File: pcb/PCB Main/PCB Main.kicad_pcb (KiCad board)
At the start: 4 copper layers, 64.1 x 56.5 mm, 82 parts, among them CN1 Conn_01x07, CN2 Conn_01x02, CN3 Conn_01x02, CN4 Conn_01x04, CN5 Conn_01x04, CN6 Conn_01x03, CN7 Conn_01x03, CN8 Conn_01x03, CN9 Conn_01x02, J1 Conn_01x03, Q1 AO3401A, SW1 SW_Reset, U1 STM32WB55RGVx, U2 AEM10941, U3 INA3221, U4 MB85RS256B, X1 32MHz, X2 32.768kHz

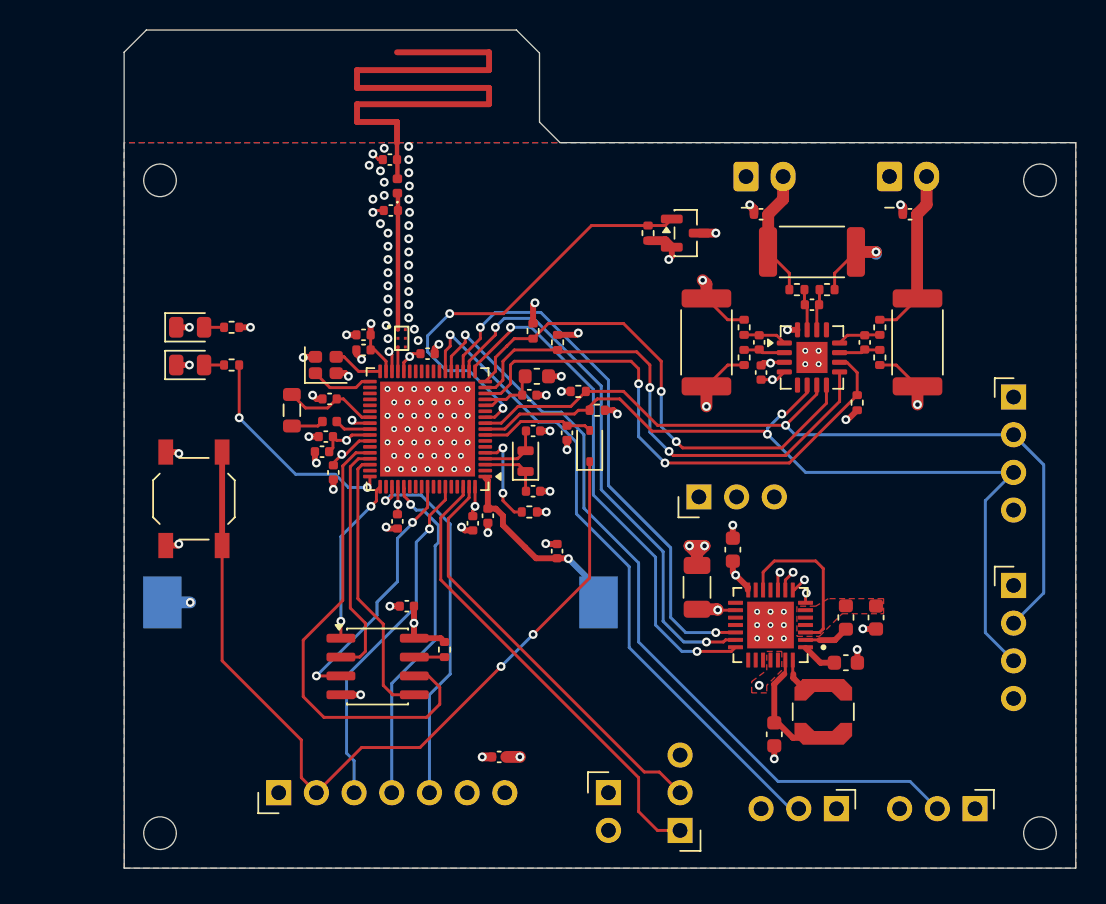
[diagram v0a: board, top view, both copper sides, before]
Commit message: islas cristales
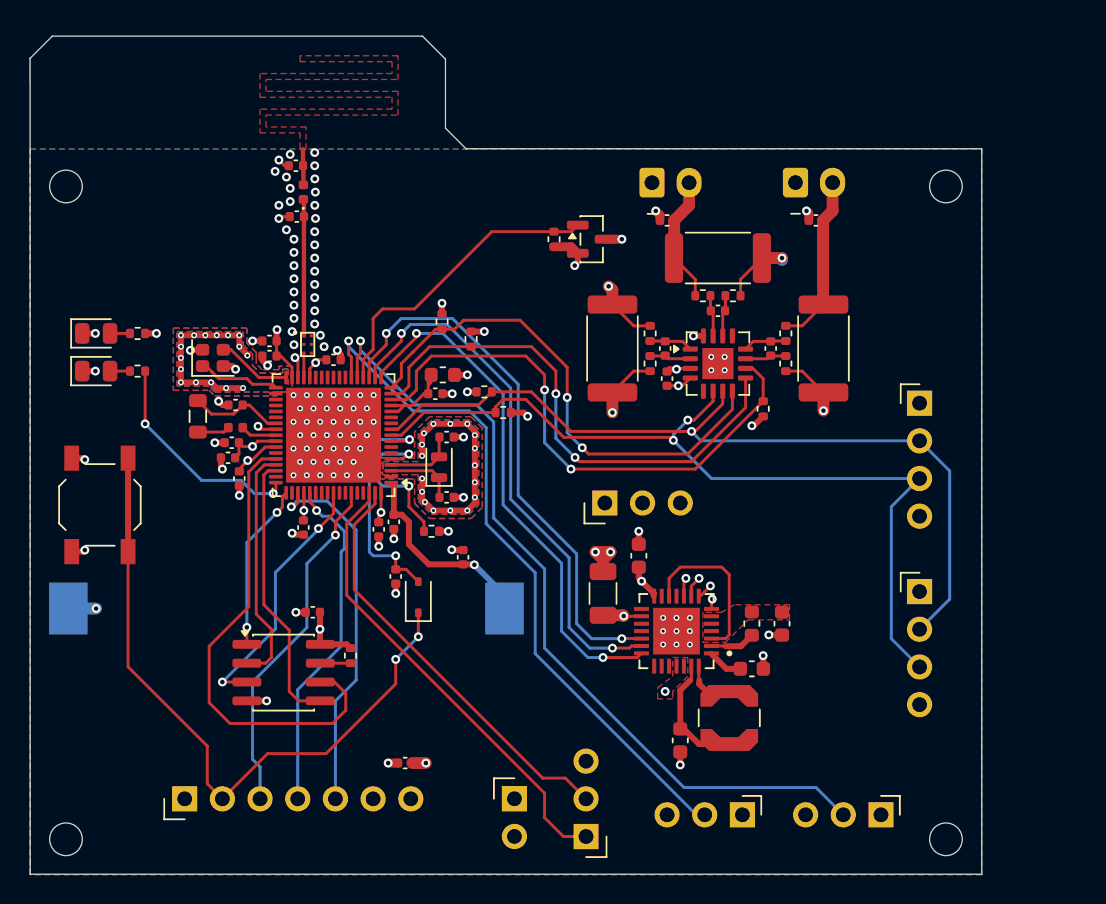
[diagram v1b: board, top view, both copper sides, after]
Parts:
- moved D1 15.4 mm to (41.0, 52.2)
- moved C23 15.1 mm to (39.5, 50.8)
- moved X1 7.62 mm to (27.2, 36.1)
- moved R13 6.72 mm to (41.9, 47.8)
- moved C18 6.35 mm to (33.3, 47.5)
- moved C2 6.35 mm to (64.8, 35.5)
- moved CN4 6.35 mm to (74.8, 39.1)
- moved CN6 6.35 mm to (72.2, 66.9)
- moved CN7 6.35 mm to (62.9, 66.9)
- moved FLT1 6.35 mm to (33.6, 35.2)
- moved H3 6.35 mm to (76.6, 68.5)
- moved R1 6.35 mm to (68.3, 35.5)
- moved BT1 6.35 mm to (32.1, 53.0)
- moved C1 6.35 mm to (57.8, 37.5)
- moved C12 6.35 mm to (38.4, 47.7)
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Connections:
- U1 pad 11: GATE_SENS -> unconnected-(U1-PC2-Pad11)
- U1 pad 21: unconnected-(U1-PA6-Pad21) -> GATE_SENS
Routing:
- net /RF/ANT: track 44.1 -> 2.42 mm
- net GND: track 40.1 -> 68.7 mm, vias 134 -> 164
- net NRST: track 57.8 -> 45.9 mm
- net GATE_SENS: track 29.1 -> 20.7 mm, vias 2 -> 0
- net Net-(D1-A): track 7.66 -> 15.8 mm, vias 0 -> 2
- net /STM32WB55RG/BOOT0: track 6.47 -> 10.8 mm
- net DFR0198: track 53.9 -> 55.7 mm
- net SEN0308: track 45.3 -> 47.0 mm
- net /STM32WB55RG/HSE_OUT: track 3.36 -> 5.00 mm
- net /STM32WB55RG/HSE_IN: track 4.24 -> 5.55 mm
- net +3.3V: track 47.0 -> 46.0 mm
- net PV_INA: track 37.1 -> 37.8 mm
- net CRI_INA: track 34.8 -> 35.3 mm
- net WAR_INA: track 33.7 -> 34.2 mm
- net VBAT_BACKUP: track 13.1 -> 13.7 mm
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- added copper zone on F.Cu, net /RF/ANT
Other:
- board text added: "islas cristales - OK plano 3.3V aislado de antena - OK vias debajo pads GND micros - OK antena como zona, no pista - OK cambiar pila holder optimizar pistas poner comentarios silkscreen"
